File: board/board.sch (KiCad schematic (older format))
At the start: 45 parts, among them Q1 FDV305N, Q2 FDV305N, Q3 FDV305N, U1 STM32F405RGTx, U2 LTC3622-23_5, Y1 16MHz

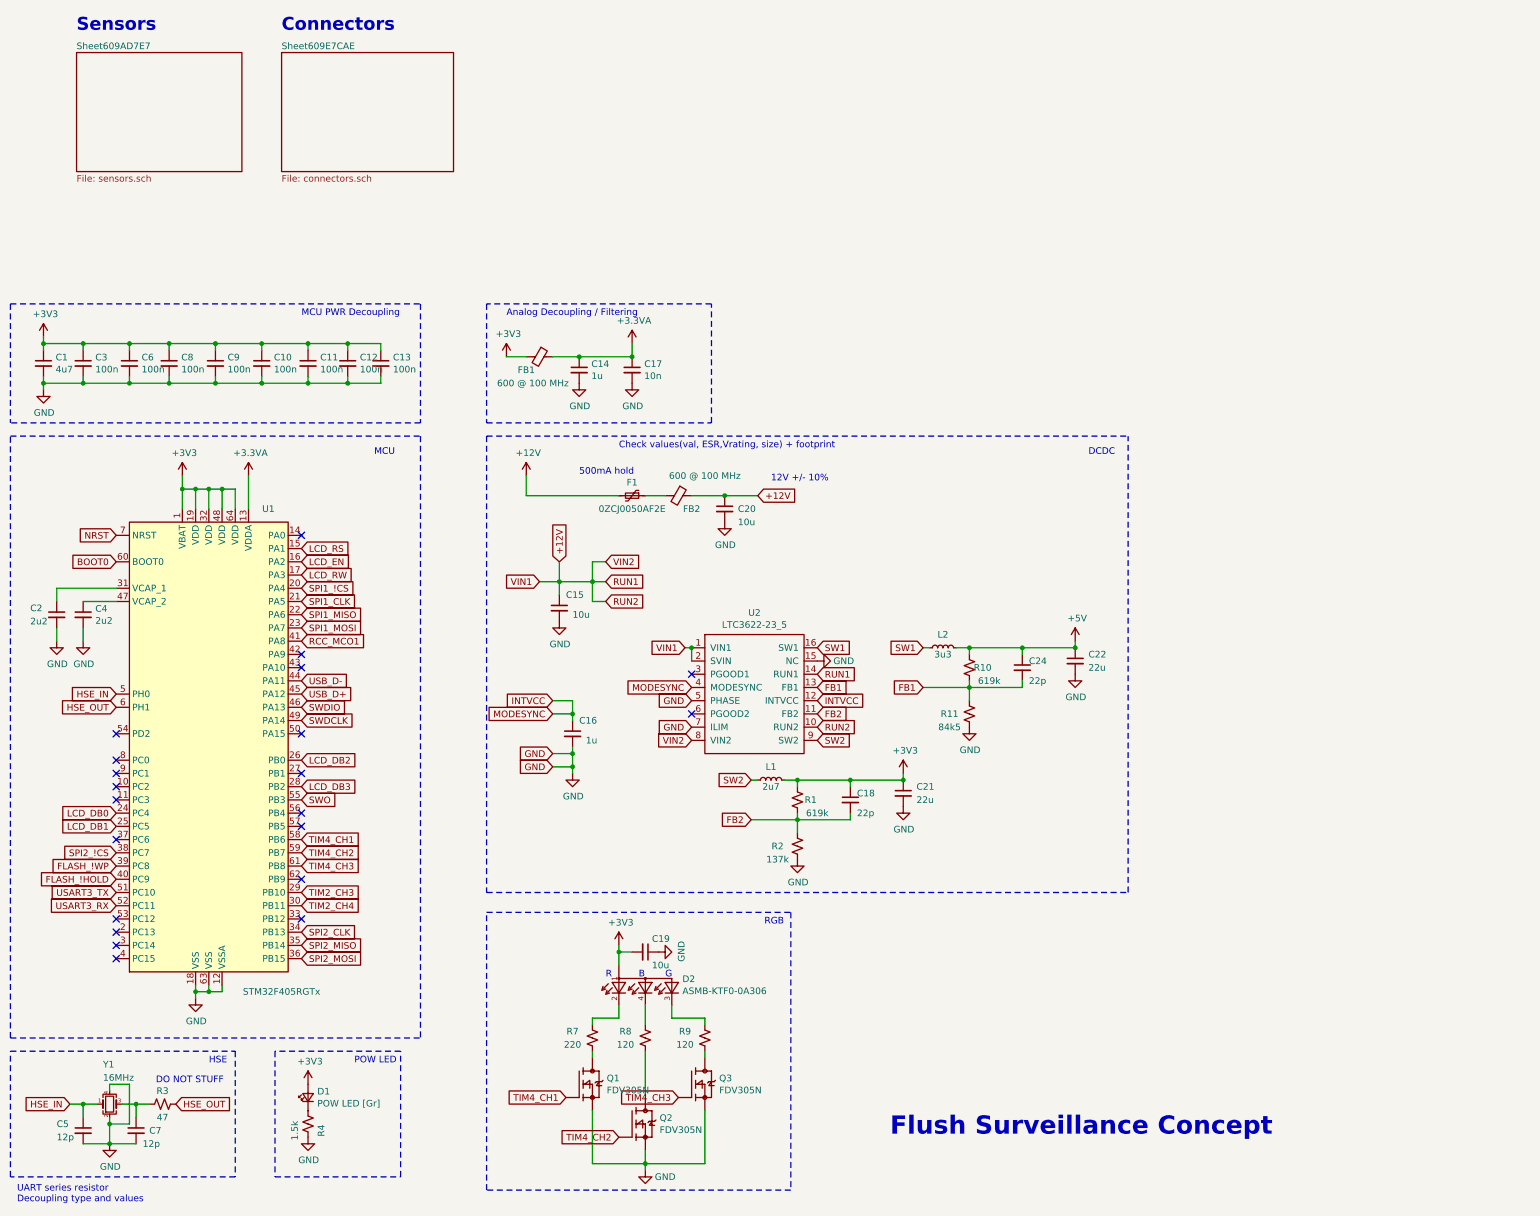
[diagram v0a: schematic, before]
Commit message: Take 2
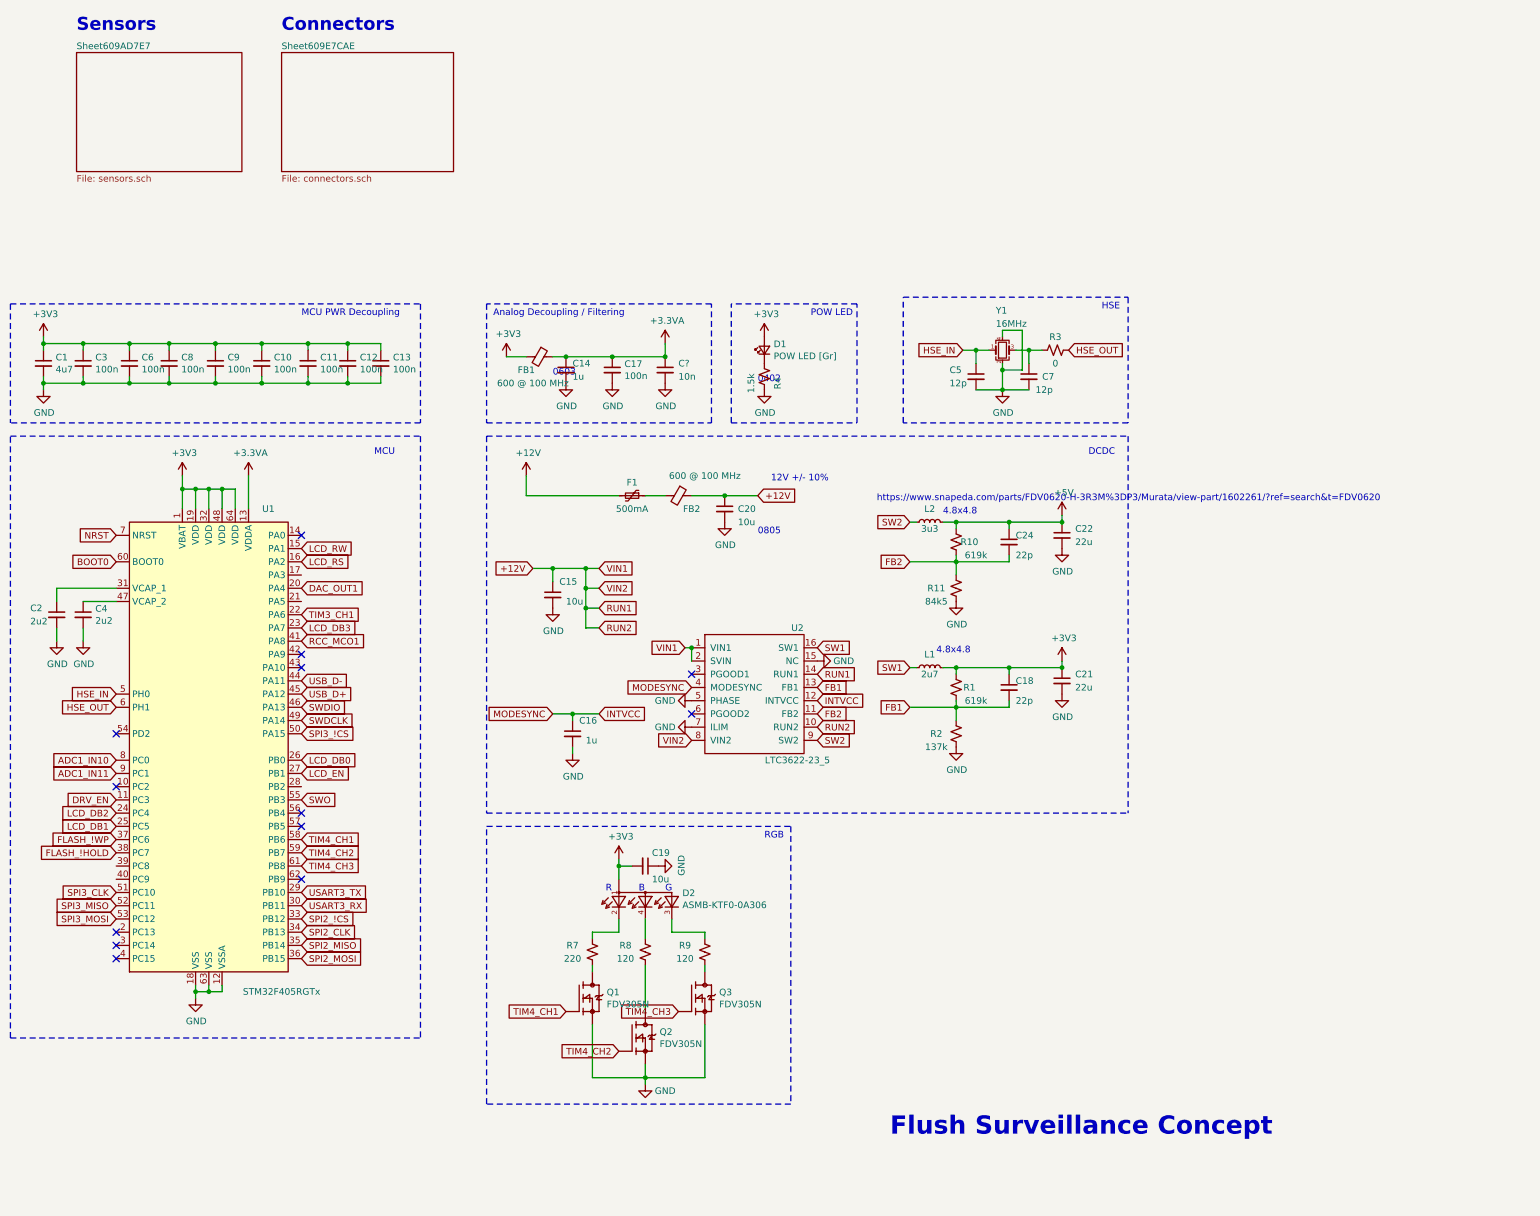
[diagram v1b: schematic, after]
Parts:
- added C?: 10n, Capacitor_SMD:C_0402_1005Metric, symbol Device:C_Small
- C17: value 10n -> 100n
- F1: value 0ZCJ0050AF2E -> 500mA
- R3: value 47 -> 0
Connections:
- net SPI1_MOSI is gone; now on net LCD_DB3: U1.23 (PA7)
- net TIM2_CH3 is gone; now on net USART3_TX: U1.29 (PB10)
- net TIM2_CH4 is gone; now on net USART3_RX: U1.30 (PB11)
- net +3.3VA: now also C?.1
- net FB1: now also C18.2, R1.1, R2.2; no longer C24.2, R10.1, R11.2
- net FB2: now also C24.2, R10.1, R11.2; no longer C18.2, R1.1, R2.2
- net FLASH_!HOLD: now also U1.38 (PC7); no longer U1.40 (PC9)
- net FLASH_!WP: now also U1.37 (PC6); no longer U1.39 (PC8)
- net GND: now also C?.2
- net LCD_DB0: now also U1.26 (PB0); no longer U1.24 (PC4)
- net LCD_DB2: now also U1.24 (PC4); no longer U1.26 (PB0)
- net LCD_DB3: no longer U1.28 (PB2)
- net LCD_EN: now also U1.27 (PB1); no longer U1.16 (PA2)
- net LCD_RS: now also U1.16 (PA2); no longer U1.15 (PA1)
- net LCD_RW: now also U1.15 (PA1); no longer U1.17 (PA3)
- net SPI2_!CS: now also U1.33 (PB12); no longer U1.38 (PC7)
- net SW1: now also L1.1; no longer L2.1
- net SW2: now also L2.1; no longer L1.1
- net USART3_RX: no longer U1.52 (PC11)
- net USART3_TX: no longer U1.51 (PC10)
- net DRV_EN: now reaches U1.11 (PC3)
- net SPI3_!CS: now reaches U1.50 (PA15)
- net SPI3_MOSI: now reaches U1.53 (PC12)
- net ADC1_IN10: now reaches U1.8 (PC0)
- net ADC1_IN11: now reaches U1.9 (PC1)
- net SPI1_!CS renamed DAC_OUT1
- net SPI1_CLK: no longer names the net of U1.21 (PA5)
- net SPI1_MISO renamed TIM3_CH1
- new net SPI3_CLK: U1.51 (PC10)
- new net SPI3_MISO: U1.52 (PC11)
- no-connect marks 21 -> 13
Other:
- note added: "0402"
- note added: "0603\n"
- note added: "0805\n"
- note added: "4.8x4.8"
- note added: "https://www.snapeda.com/parts/FDV0620-H-3R3M%3DP3/Murata/view-part/1602261/?ref=search&t=FDV0620"
- note removed: "500mA hold\n"
- note removed: "Check values(val, ESR,Vrating, size) + footprint"
- note removed: "DO NOT STUFF\n"
- note removed: "UART series resistor\nDecoupling type and values"
- moved on the sheet: C14, C15, C17, C18, C19, C21, C22, C24, C5, C7, D1, D2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
